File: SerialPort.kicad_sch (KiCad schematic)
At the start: 9 parts, among them J4 DB9_Male, U15 MC6850, U16 MAX232, U19 74HCT92

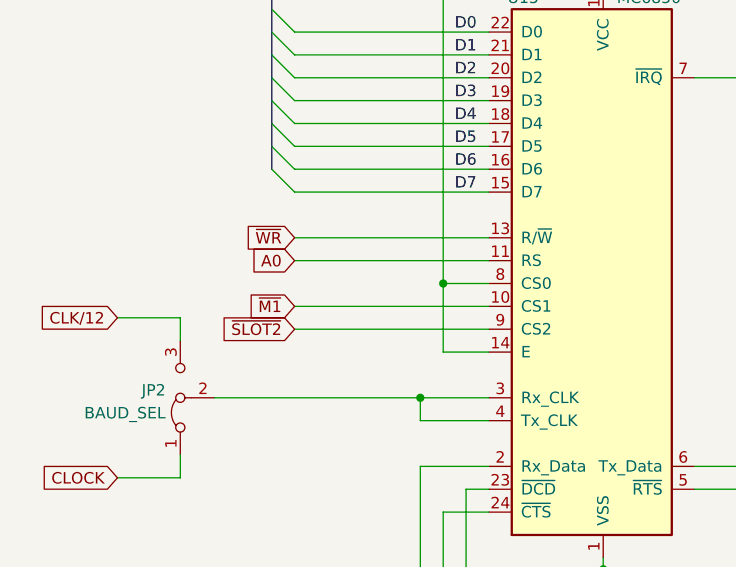
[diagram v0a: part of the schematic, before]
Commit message: Work-in-progress
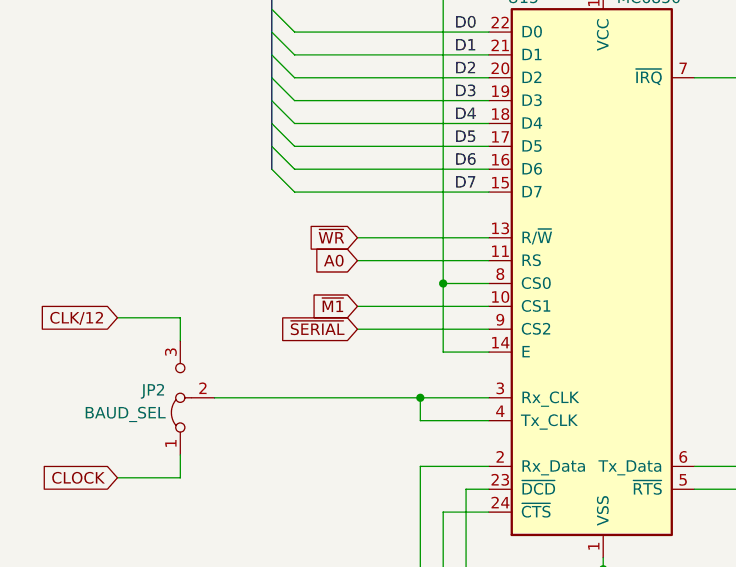
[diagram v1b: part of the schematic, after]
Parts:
- U15: footprint Package_DIP:DIP-24_W15.24mm_LongPads -> Package_DIP:DIP-24_W15.24mm
- U16: footprint Package_DIP:DIP-16_W7.62mm_LongPads -> Package_DIP:DIP-16_W7.62mm
- U19: footprint Package_DIP:DIP-14_W7.62mm_LongPads -> Package_DIP:DIP-14_W7.62mm
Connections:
- net ~{SLOT2} renamed ~{SERIAL}
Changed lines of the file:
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@@
     (stroke (width 0) (type default))
   )
-  (wire (pts (xy 75.565 73.025) (xy 53.975 73.025))
+  (wire (pts (xy 75.565 73.025) (xy 60.96 73.025))
     (stroke (width 0) (type default))
   )
@@
     (stroke (width 0) (type default))
   )
-  (wire (pts (xy 75.565 80.645) (xy 53.975 80.645))
+  (wire (pts (xy 75.565 80.645) (xy 60.96 80.645))
     (stroke (width 0) (type default))
   )
@@
     (stroke (width 0) (type default))
   )
-  (wire (pts (xy 53.975 83.185) (xy 75.565 83.185))
+  (wire (pts (xy 60.96 83.185) (xy 75.565 83.185))
     (stroke (width 0) (type default))
   )
@@
     (stroke (width 0) (type default))
   )
-  (wire (pts (xy 75.565 75.565) (xy 53.975 75.565))
+  (wire (pts (xy 75.565 75.565) (xy 60.96 75.565))
     (stroke (width 0) (type default))
   )
@@
     )
   )
-  (global_label "~{M1}" (shape input) (at 53.975 80.645 180) (fields_autoplaced)
+  (global_label "~{M1}" (shape input) (at 60.96 80.645 180) (fields_autoplaced)
     (effects (font (size 1.27 1.27)) (justify right))
-    (property "Intersheetrefs" "${INTERSHEET_REFS}" (at 1.905 -26.035 0)
-      (effects (font (size 1.27 1.27)) hide)
+    (property "Intersheetrefs" "${INTERSHEET_REFS}" (at 8.89 -26.035 0)
+      (effects (font (size 1.27 1.27)) hide)
+    )
+  )
+  (global_label "~{SERIAL}" (shape input) (at 60.96 83.185 180) (fields_autoplaced)
+    (effects (font (size 1.27 1.27)) (justify right))
+    (property "Intersheetrefs" "${INTERSHEET_REFS}" (at 51.882 83.185 0)
+      (effects (font (size 1.27 1.27)) (justify right) hide)
     )
   )
@@
     )
   )
-  (global_label "A0" (shape input) (at 53.975 75.565 180) (fields_autoplaced)
+  (global_label "A0" (shape input) (at 60.96 75.565 180) (fields_autoplaced)
     (effects (font (size 1.27 1.27)) (justify right))
-    (property "Intersheetrefs" "${INTERSHEET_REFS}" (at 1.905 -27.305 0)
-      (effects (font (size 1.27 1.27)) hide)
-    )
-  )
-  (global_label "~{WR}" (shape input) (at 53.975 73.025 180) (fields_autoplaced)
+    (property "Intersheetrefs" "${INTERSHEET_REFS}" (at 8.89 -27.305 0)
+      (effects (font (size 1.27 1.27)) hide)
+    )
+  )
+  (global_label "~{WR}" (shape input) (at 60.96 73.025 180) (fields_autoplaced)
     (effects (font (size 1.27 1.27)) (justify right))
-    (property "Intersheetrefs" "${INTERSHEET_REFS}" (at 1.905 -26.035 0)
+    (property "Intersheetrefs" "${INTERSHEET_REFS}" (at 8.89 -26.035 0)
       (effects (font (size 1.27 1.27)) hide)
     )
@@
     )
   )
-  (global_label "~{SLOT2}" (shape input) (at 53.975 83.185 180) (fields_autoplaced)
-    (effects (font (size 1.27 1.27)) (justify right))
-    (property "Intersheetrefs" "${INTERSHEET_REFS}" (at 45.9056 83.1056 0)
-      (effects (font (size 1.27 1.27)) (justify right) hide)
-    )
-  )
   (symbol (lib_id "Interface_UART:MC6850") (at 88.265 78.105 0) (unit 1)
     (in_bom yes) (on_board yes) (dnp no)
@@
       (effects (font (size 1.27 1.27)))
     )
-    (property "Footprint" "Package_DIP:DIP-24_W15.24mm_LongPads" (at 89.535 107.315 0)
+    (property "Footprint" "Package_DIP:DIP-24_W15.24mm" (at 89.535 107.315 0)
       (effects (font (size 1.27 1.27)) (justify left) hide)
     )
@@
       (effects (font (size 1.27 1.27)))
     )
-    (property "Footprint" "Package_DIP:DIP-16_W7.62mm_LongPads" (at 159.385 117.475 0)
+    (property "Footprint" "Package_DIP:DIP-16_W7.62mm" (at 159.385 117.475 0)
       (effects (font (size 1.27 1.27)) (justify left) hide)
     )
@@
       (effects (font (size 1.27 1.27)) (justify left))
     )
-    (property "Footprint" "Package_DIP:DIP-14_W7.62mm_LongPads" (at 76.835 170.18 0)
-      (effects (font (size 1.27 1.27)) hide)
-    )
+    (property "Footprint" "Package_DIP:DIP-14_W7.62mm" (at 76.835 170.18 0)
+      (effects (font (size 1.27 1.27)) hide)
+    )
